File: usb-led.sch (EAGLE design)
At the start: 13 parts, among them U1 ATtiny85-20SU

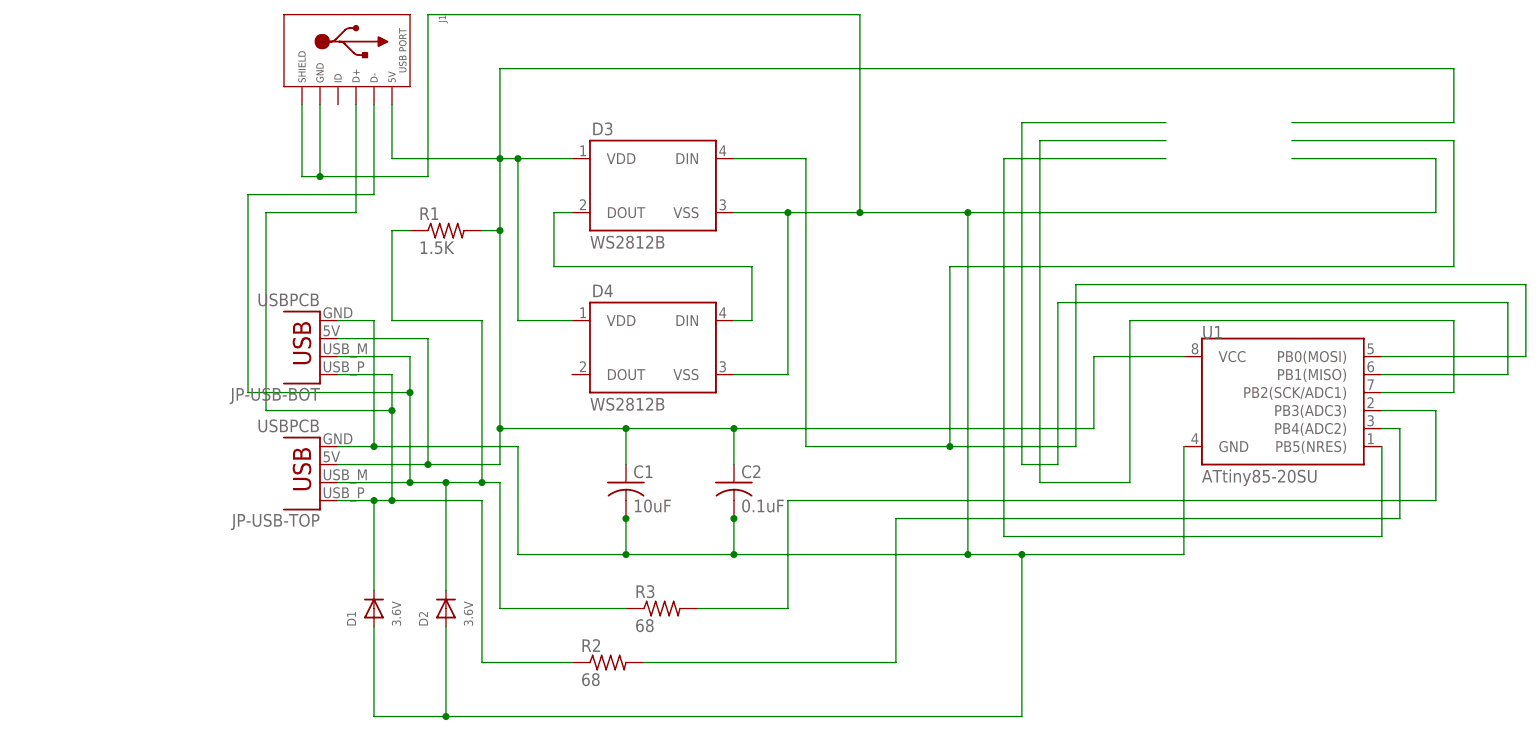
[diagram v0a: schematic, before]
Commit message: mf2.
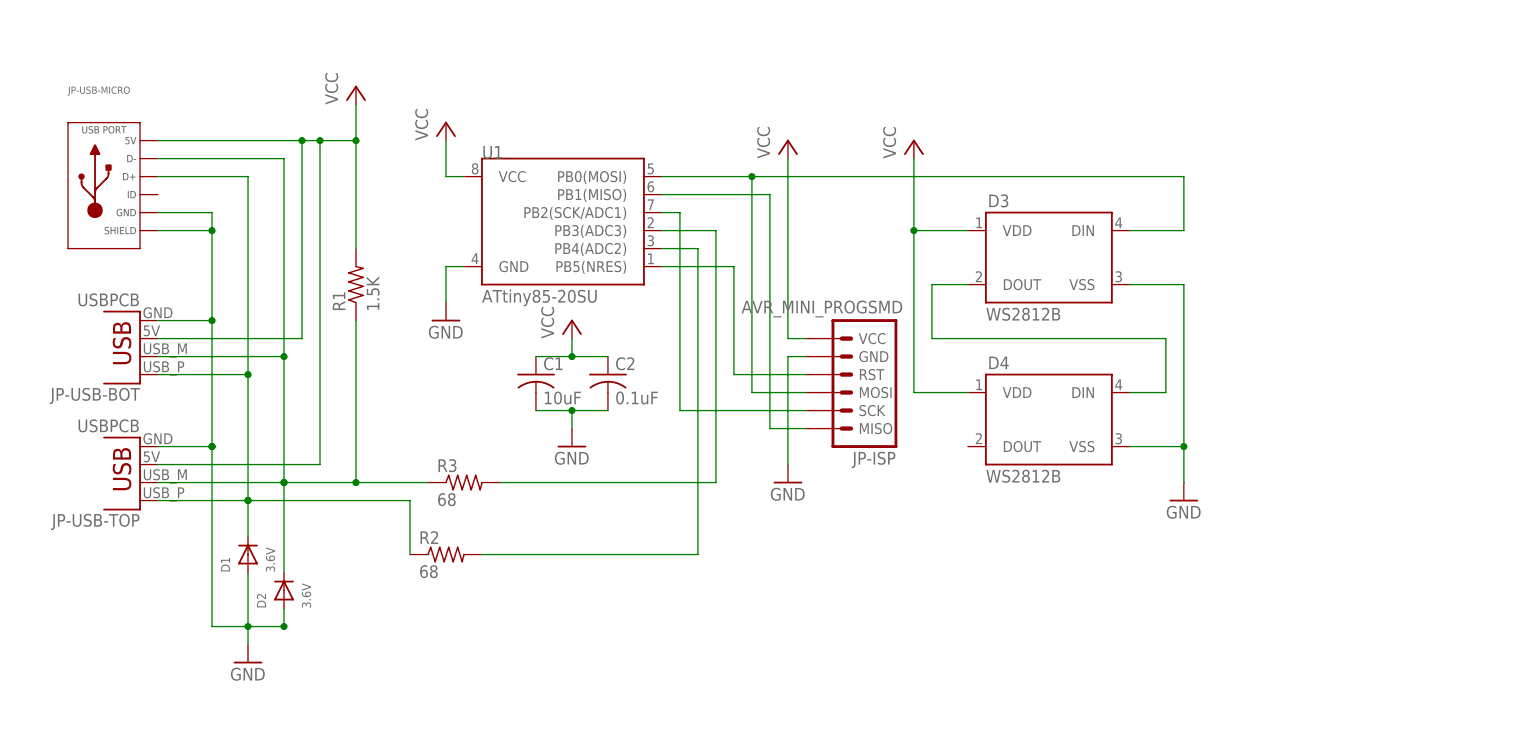
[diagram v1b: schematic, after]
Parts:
- removed J1: (no value), MF_Connectors:USB_MICRO_RIGHT
- added JP-ISP: AVR_MINI_PROGSMD, SparkFun-Connectors:AVR_MINI_PROGSMD
- added JP-USB-MICRO: (no value), MF_Connectors:USB_MICRO_RIGHT
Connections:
- net GND: now also JP-ISP.GND, JP-USB-MICRO.GND, JP-USB-MICRO.SLD; no longer J1.GND, J1.SLD
- net MISO: now also JP-ISP.MISO
- net MOSI/DIN: now also JP-ISP.MOSI
- net RESET: now also JP-ISP.RST
- net SCK: now also JP-ISP.SCK
- net USB_D_MINUS_RAW: now also JP-USB-MICRO.D-; no longer J1.D-
- net USB_D_PLUS_RAW: now also JP-USB-MICRO.D+; no longer J1.D+
- net VCC: now also JP-ISP.VCC, JP-USB-MICRO.5V; no longer J1.5V
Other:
- moved on the sheet: C1, C2, D1, D2, D3, D4, JP-USB-BOT, JP-USB-TOP, R1, R2, R3, U1
